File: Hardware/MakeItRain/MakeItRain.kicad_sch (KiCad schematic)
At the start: 16 parts, among them J1 Conn_02x14_Odd_Even, J2 Conn_02x19_Odd_Even, J3 Conn_01x19, J6 Adafruit_DS3231, U1 MCP23008-xP

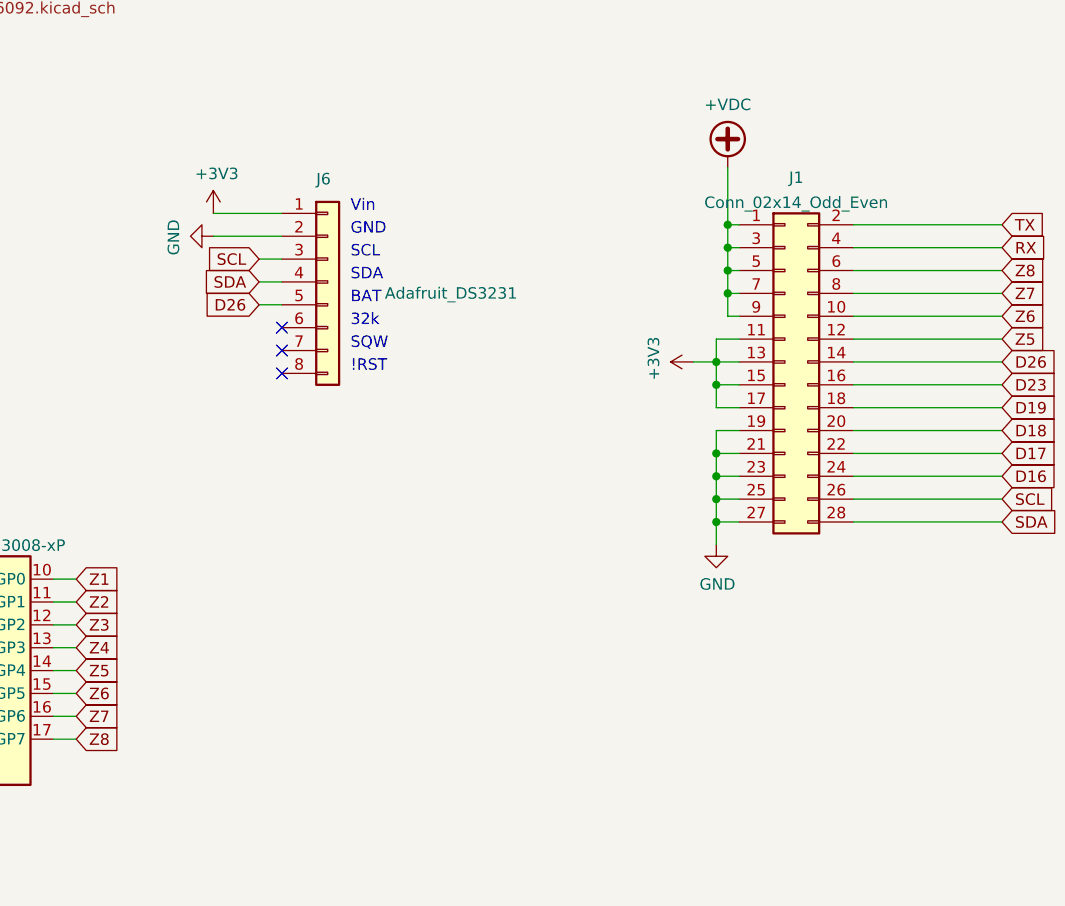
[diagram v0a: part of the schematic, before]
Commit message: wip
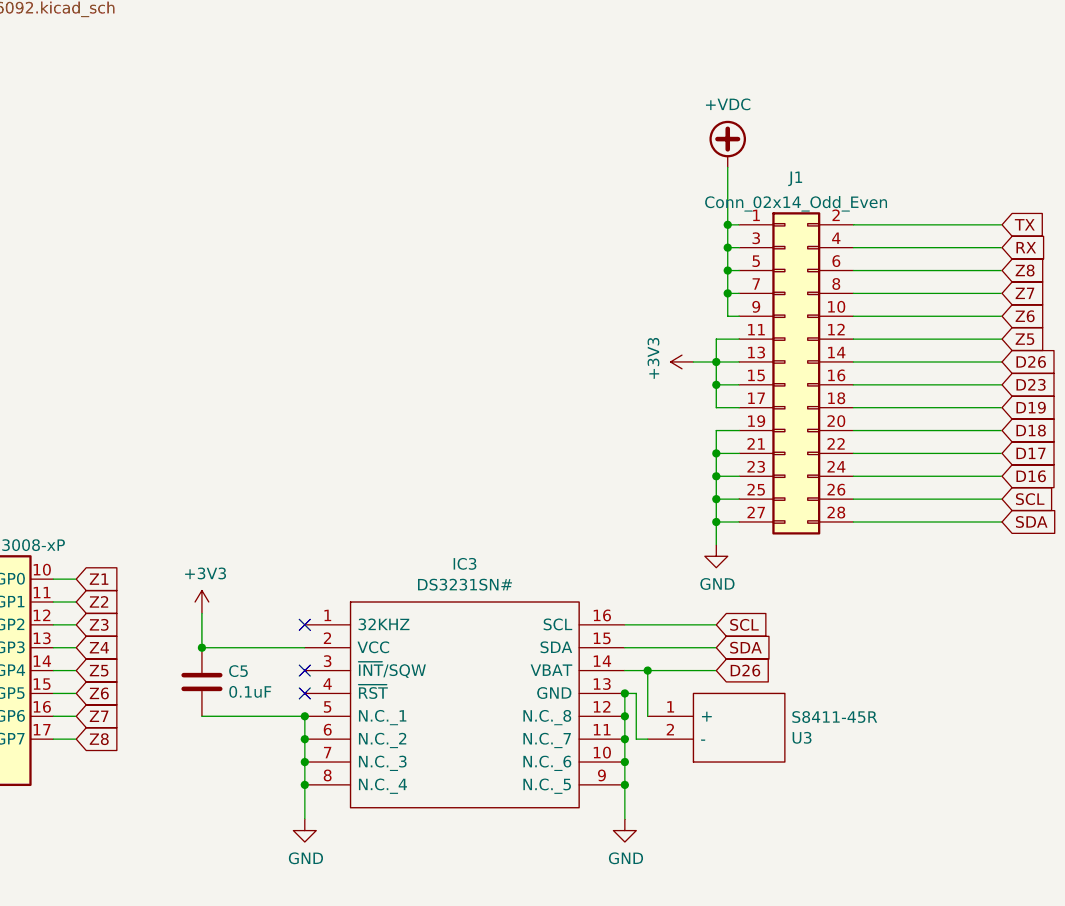
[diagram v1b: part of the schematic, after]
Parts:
- removed J6: Adafruit_DS3231, Connector_PinHeader_1.00mm:PinHeader_1x08_P1.00mm_Vertical_SMD_Pin1Right, symbol Connector_Generic:Conn_01x08
- added C5: 0.1uF, Capacitor_THT:C_Rect_L9.0mm_W3.6mm_P7.50mm_MKT, symbol Device:C
- added IC3: DS3231SN#, SamacSys_Parts:SOIC127P1032X265-16N, symbol SamacSys_Parts:DS3231SN#
- added U3: S8411-45R, SamacSys_Parts:S8411-45R_1, symbol SamacSys_Parts:S8411-45R
- R3, R36, R37, R38, R4: footprint Resistor_THT:R_Axial_DIN0207_L6.3mm_D2.5mm_P2.54mm_Vertical -> Resistor_SMD:R_1206_3216Metric_Pad1.30x1.75mm_HandSolder
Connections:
- net +3V3: now also C5.1, IC3.2 (VCC)
- net D21: now also IC3.15 (SDA)
- net D22: now also IC3.16 (SCL)
- net D26: now also IC3.14 (VBAT), U3.1 (+)
- net GND: now also C5.2, IC3.10 (N.C._6), IC3.11 (N.C._7), IC3.12 (N.C._8), IC3.13 (GND), IC3.5 (N.C._1), IC3.6 (N.C._2), IC3.7 (N.C._3), IC3.8 (N.C._4), IC3.9 (N.C._5), U3.2 (-)
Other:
- note removed: "!RST"
- note removed: "32k"
- note removed: "BAT"
- note removed: "GND"
- note removed: "SCL"
- note removed: "SDA"
- note removed: "SQW"
- note removed: "Vin"
